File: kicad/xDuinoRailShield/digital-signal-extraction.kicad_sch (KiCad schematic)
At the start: 11 parts, among them Q1 T2N7002BK, U3 6N137, U4 EL817

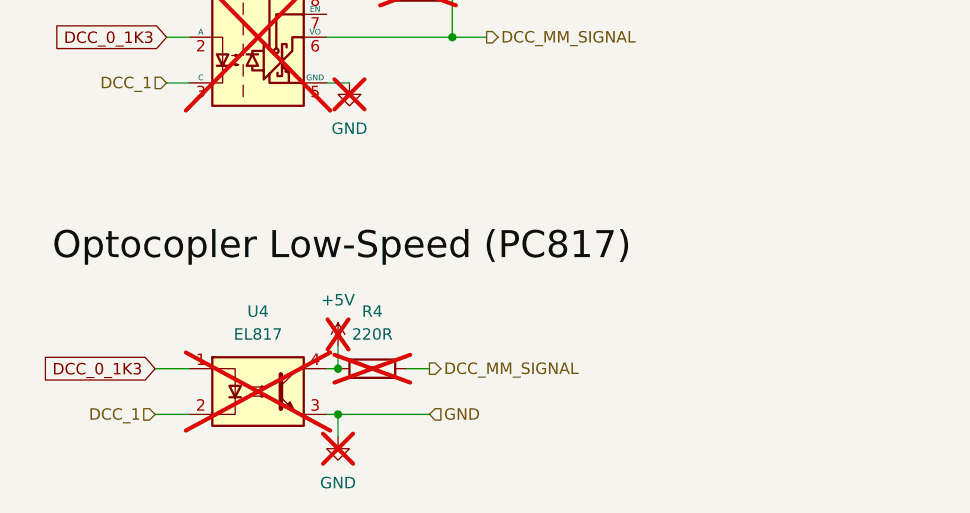
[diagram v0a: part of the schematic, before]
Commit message: More nice changes
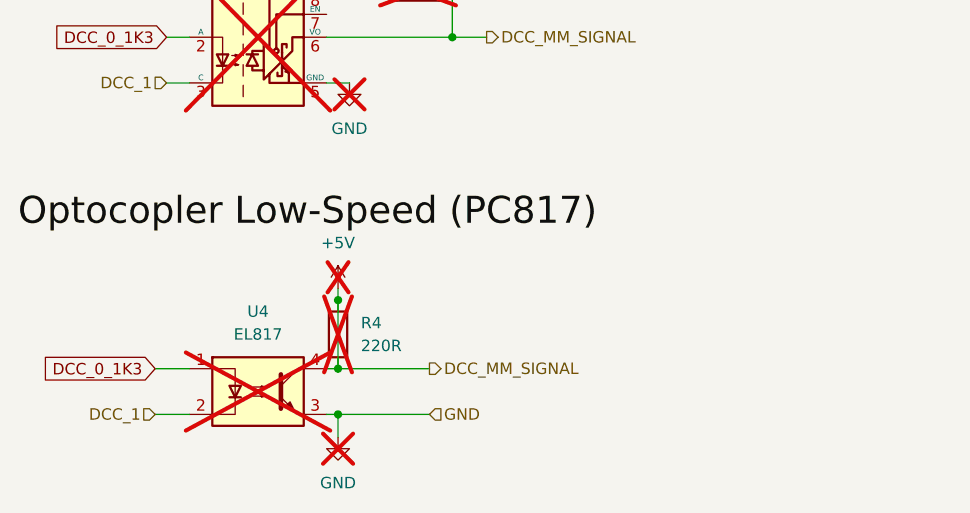
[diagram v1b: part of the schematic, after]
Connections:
- net DCC_MM_SIGNAL is gone; now on net +5V: Q1.3 (D), R4.1, R5.1, R5.2, U3.6 (VO)
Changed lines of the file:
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@@
 	(paper "A4")
+	(junction
+		(at 74.93 140.97)
+		(diameter 0)
+		(color 0 0 0 0)
+	)
 	(junction
 		(at 68.58 71.12)
@@
 	)
 	(junction
+		(at 74.93 148.59)
+		(diameter 0)
+		(color 0 0 0 0)
+	)
+	(junction
 		(at 166.37 87.63)
 		(diameter 0)
@@
 	)
 	(junction
-		(at 74.93 148.59)
-		(diameter 0)
-		(color 0 0 0 0)
-	)
-	(junction
 		(at 166.37 90.17)
 		(diameter 0)
@@
 	(wire
 		(pts
-			(xy 74.93 146.05) (xy 74.93 148.59)
+			(xy 74.93 140.97) (xy 74.93 148.59)
 		)
 		(stroke
@@
 	(wire
 		(pts
+			(xy 74.93 139.7) (xy 74.93 140.97)
+		)
+		(stroke
+			(width 0)
+			(type default)
+		)
+	)
+	(wire
+		(pts
 			(xy 74.93 156.21) (xy 74.93 153.67)
 		)
@@
 	(wire
 		(pts
-			(xy 82.55 148.59) (xy 85.09 148.59)
+			(xy 74.93 148.59) (xy 85.09 148.59)
 		)
 		(stroke
@@
 	)
 	(label "Optocopler Low-Speed (PC817)"
-		(at 43.18 137.16 0)
+		(at 39.37 133.35 0)
 		(fields_autoplaced yes)
 		(effects
@@
 		(lib_name "+5V_1")
 		(lib_id "power:+5V")
-		(at 74.93 146.05 0)
+		(at 74.93 139.7 0)
 		(unit 1)
 		(exclude_from_sim no)
@@
 		(fields_autoplaced yes)
 		(property "Reference" "#PWR019"
-			(at 74.93 149.86 0)
+			(at 74.93 143.51 0)
 			(effects
 				(font
@@
 		)
 		(property "Value" "+5V"
-			(at 74.93 140.97 0)
+			(at 74.93 134.62 0)
 			(effects
 				(font
@@
 		)
 		(property "Footprint" ""
-			(at 74.93 146.05 0)
+			(at 74.93 139.7 0)
 			(effects
 				(font
@@
 		)
 		(property "Datasheet" ""
-			(at 74.93 146.05 0)
+			(at 74.93 139.7 0)
 			(effects
 				(font
@@
 		)
 		(property "Description" ""
-			(at 74.93 146.05 0)
+			(at 74.93 139.7 0)
 			(effects
 				(font
@@
 	)
 	(symbol
-		(lib_id "Device:R")
-		(at 78.74 148.59 270)
-		(unit 1)
-		(exclude_from_sim no)
-		(in_bom yes)
-		(on_board no)
-		(dnp yes)
-		(fields_autoplaced yes)
-		(property "Reference" "R4"
-			(at 78.74 142.24 90)
-			(effects
-				(font
-					(size 1.27 1.27)
-				)
-			)
-		)
-		(property "Value" "220R"
-			(at 78.74 144.78 90)
-			(effects
-				(font
-					(size 1.27 1.27)
-				)
-			)
-		)
-		(property "Footprint" "Resistor_SMD:R_0603_1608Metric_Pad0.98x0.95mm_HandSolder"
-			(at 78.74 146.812 90)
-			(effects
-				(font
-					(size 1.27 1.27)
-				)
-				(hide yes)
-			)
-		)
-		(property "Datasheet" "~"
-			(at 78.74 148.59 0)
-			(effects
-				(font
-					(size 1.27 1.27)
-				)
-				(hide yes)
-			)
-		)
-		(property "Description" ""
-			(at 78.74 148.59 0)
-			(effects
-				(font
-					(size 1.27 1.27)
-				)
-				(hide yes)
-			)
-		)
-		(property "LCSC" "C17557"
-			(at 78.74 148.59 0)
-			(effects
-				(font
-					(size 1.27 1.27)
-				)
-				(hide yes)
-			)
-		)
-		(pin "2"
-		)
-		(pin "1"
-		)
-		(instances
-			(project "xDuinoRailShield"
-				(path "/e63e39d7-6ac0-4ffd-8aa3-1841a4541b55/b84a333b-f29e-43df-b84d-edef752a64aa"
-					(reference "R4")
-					(unit 1)
-				)
-			)
-		)
-	)
-	(symbol
 		(lib_id "Device:C")
 		(at 68.58 67.31 0)
@@
 					(unit 1)
 				)
+			)
+		)
+	)
+	(symbol
+		(lib_id "Device:R")
+		(at 74.93 144.78 0)
+		(unit 1)
+		(exclude_from_sim no)
+		(in_bom yes)
+		(on_board no)
+		(dnp yes)
+		(fields_autoplaced yes)
+		(property "Reference" "R4"
+			(at 77.47 143.5099 0)
+			(effects
+				(font
+					(size 1.27 1.27)
+				)
+				(justify left)
+			)
+		)
+		(property "Value" "220R"
+			(at 77.47 146.0499 0)
+			(effects
+				(font
+					(size 1.27 1.27)
+				)
+				(justify left)
+			)
+		)
+		(property "Footprint" "Resistor_SMD:R_0603_1608Metric_Pad0.98x0.95mm_HandSolder"
+			(at 73.152 144.78 90)
+			(effects
+				(font
+					(size 1.27 1.27)
+				)
+				(hide yes)
+			)
+		)
+		(property "Datasheet" "~"
+			(at 74.93 144.78 0)
+			(effects
+				(font
+					(size 1.27 1.27)
+				)
+				(hide yes)
+			)
+		)
+		(property "Description" ""
+			(at 74.93 144.78 0)
+			(effects
+				(font
+					(size 1.27 1.27)
+				)
+				(hide yes)
+			)
+		)
+		(property "LCSC" "C17557"
+			(at 74.93 144.78 0)
+			(effects
+				(font
+					(size 1.27 1.27)
+				)
+				(hide yes)
+			)
+		)
+		(pin "2"
+		)
+		(pin "1"
+		)
+		(instances
+			(project "xDuinoRailShield"
+				(path "/e63e39d7-6ac0-4ffd-8aa3-1841a4541b55/b84a333b-f29e-43df-b84d-edef752a64aa"
+					(reference "R4")
+					(unit 1)
+				)
